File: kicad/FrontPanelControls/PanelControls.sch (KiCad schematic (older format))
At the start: 35 parts, among them J1 Conn_02x04_Odd_Even, SW5 ADJ, U1 PCF8591, U2 PCF8574, U3 WS2812D, U4 WS2812D, U5 WS2812D, U6 WS2812D, U7 WS2812D, U8 WS2812D

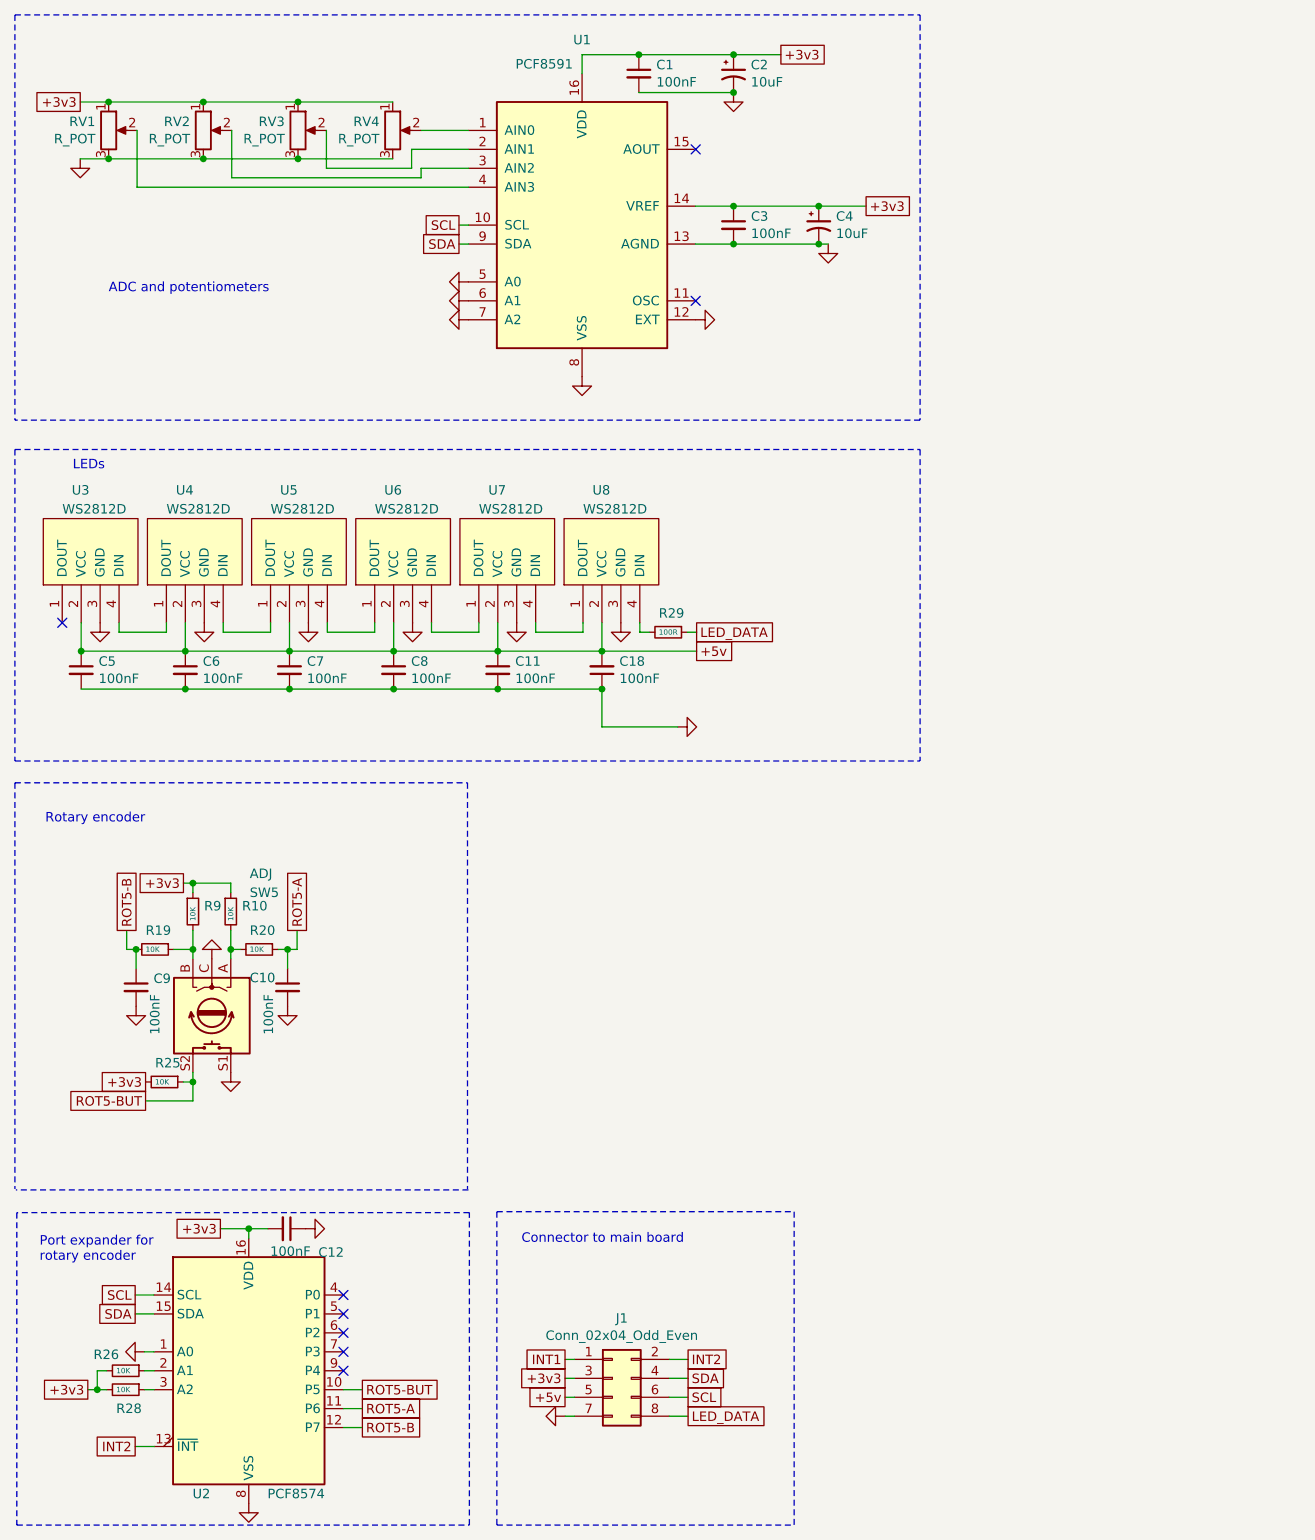
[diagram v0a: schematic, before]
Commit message: initial changes FrontPanel
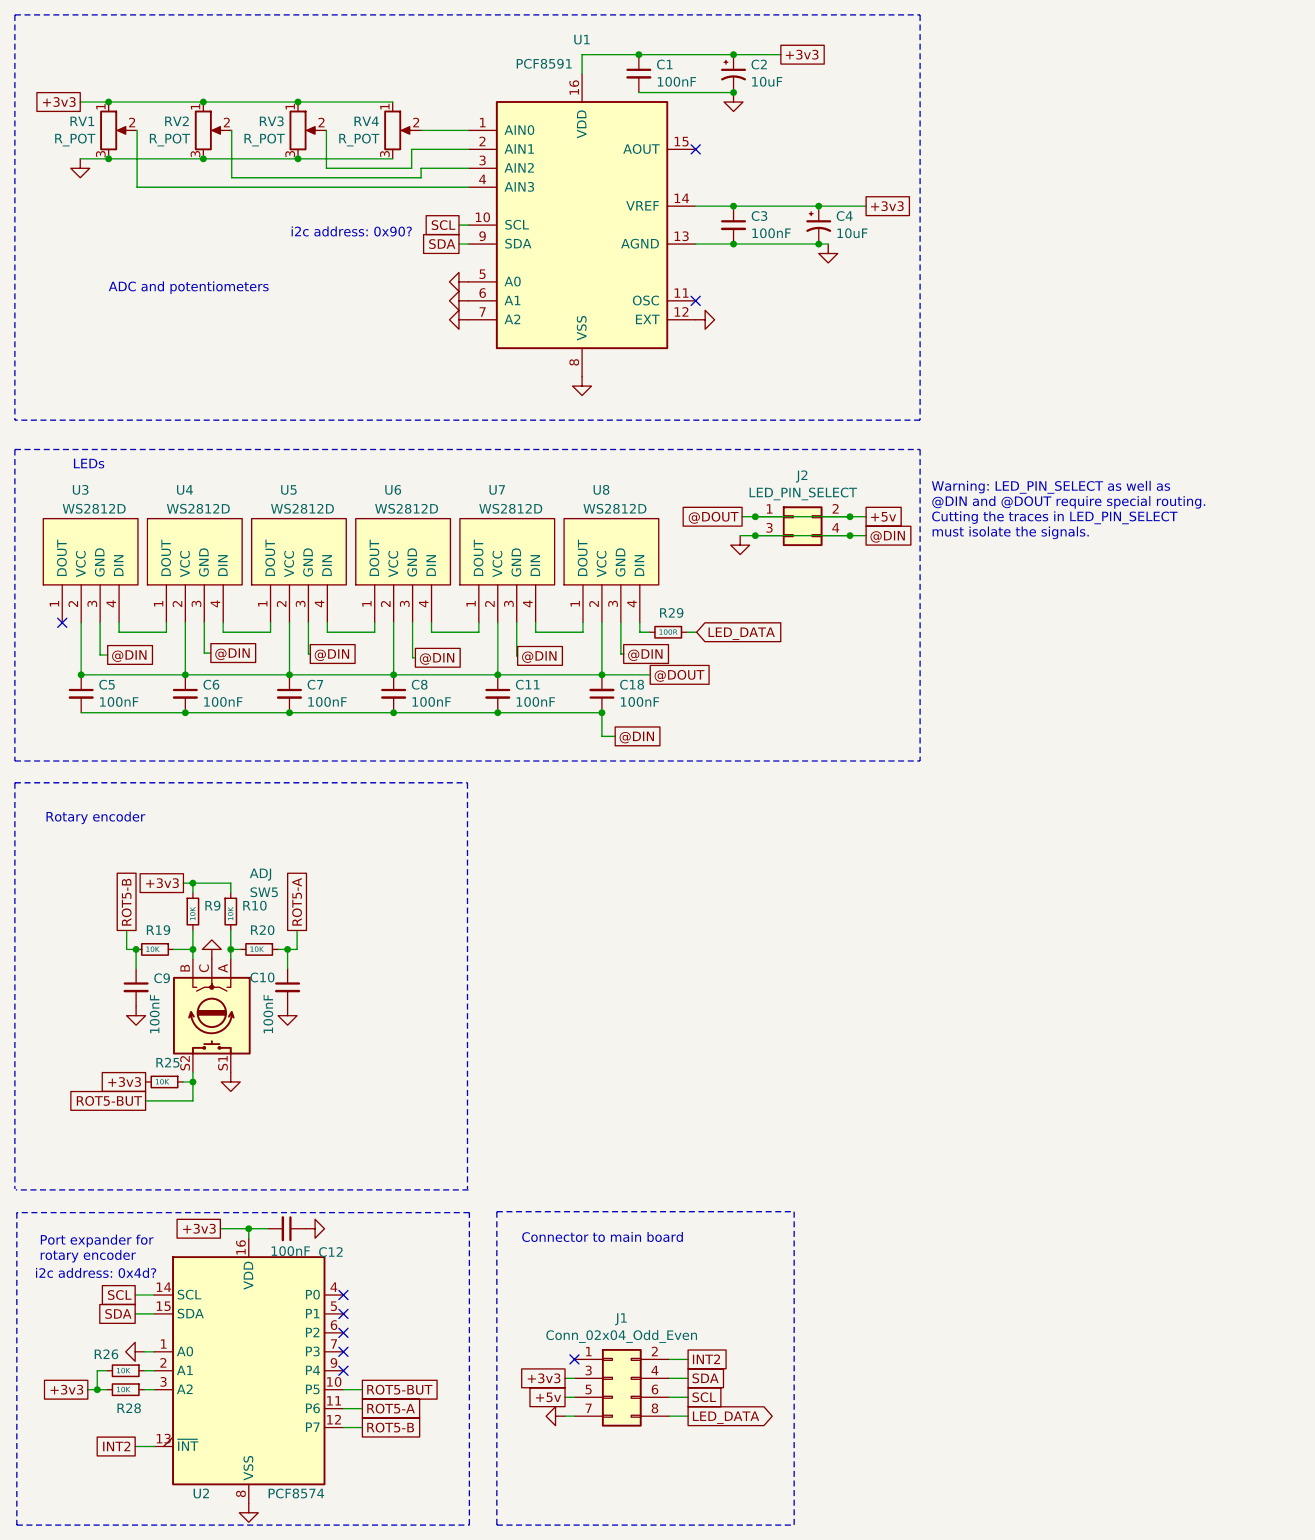
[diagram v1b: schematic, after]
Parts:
- added J2: LED_PIN_SELECT, Connector_PinHeader_2.54mm:PinHeader_2x02_P2.54mm_Vertical, symbol Connector_Generic:Conn_02x02_Odd_Even
- C4: footprint Capacitor_THT:CP_Radial_D4.0mm_P1.50mm -> Capacitor_THT:CP_Radial_D4.0mm_P2.00mm
- U1: footprint Package_SO:SOIC-16W_7.5x10.3mm_P1.27mm -> Package_SO:SO-16_5.3x10.2mm_P1.27mm
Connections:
- net +5v: now also J2.1 (Pin_1), J2.2 (Pin_2)
- net GND: now also J2.3 (Pin_3), J2.4 (Pin_4)
- net INT1: no longer names the net of J1.1 (Pin_1)
- no-connect marks 8 -> 9
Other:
- note added: "Warning: LED_PIN_SELECT as well as \n@DIN and @DOUT require special routing. \nCutting the traces in LED_PIN_SELECT \nmust isolate the signals."
- note added: "i2c address: 0x4d?\n"
- note added: "i2c address: 0x90?\n"
- moved on the sheet: C11, C18, C5, C6, C7, C8
